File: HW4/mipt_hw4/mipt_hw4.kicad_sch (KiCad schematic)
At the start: 8 parts, among them K1 Panasonic_ALFG1PF12, Q1 BC327, SW1 SW_MEC_5E

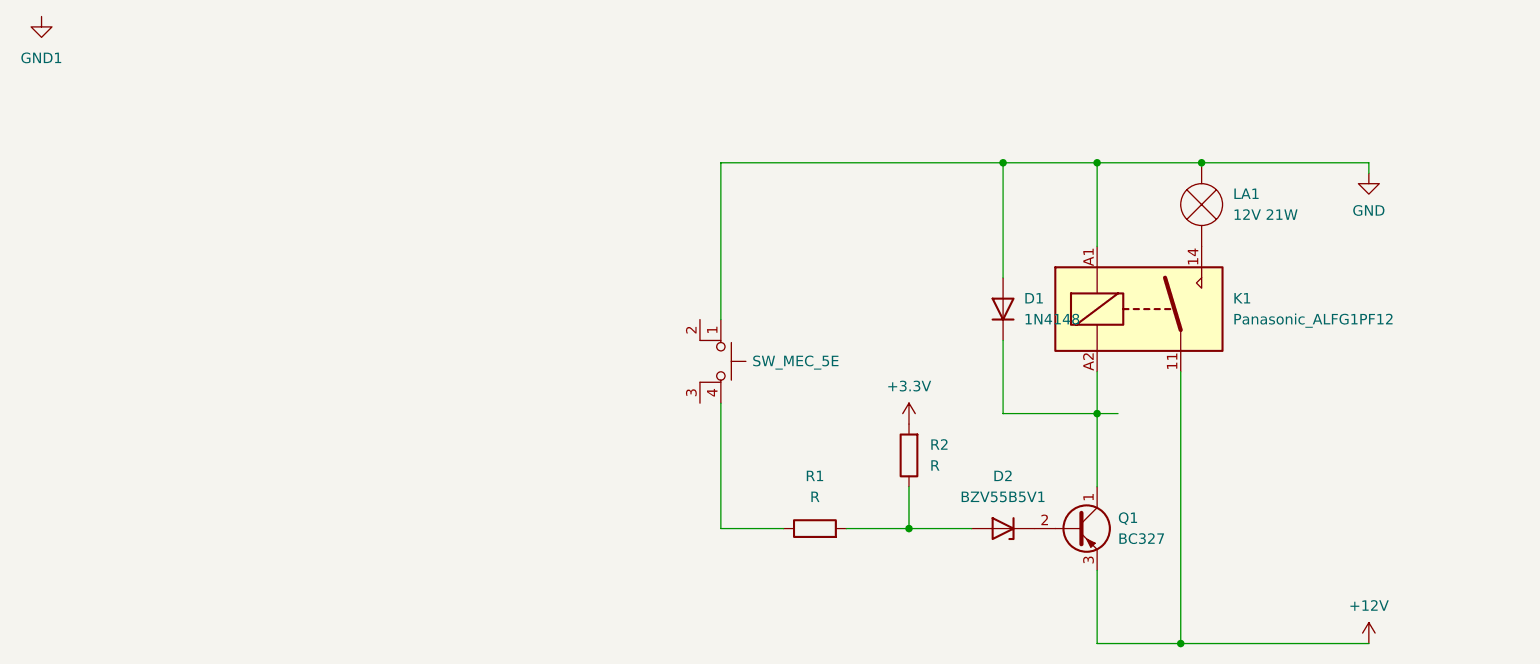
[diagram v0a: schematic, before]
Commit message: HW4 completed
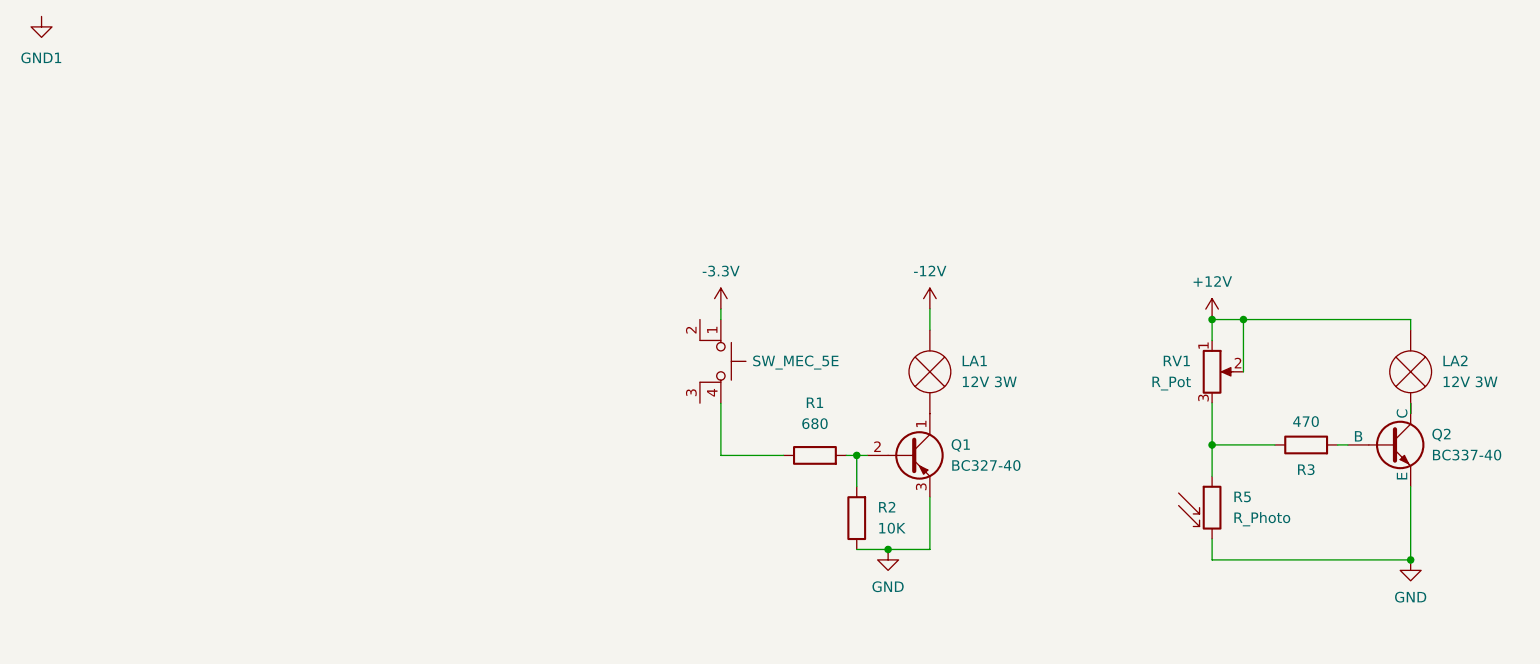
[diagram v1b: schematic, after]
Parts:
- removed D1: 1N4148, Diode_THT:D_DO-35_SOD27_P7.62mm_Horizontal, symbol Diode:1N4148
- removed D2: BZV55B5V1, Diode_SMD:D_MiniMELF, symbol Diode:BZV55B5V1
- removed K1: Panasonic_ALFG1PF12, Relay_THT:Relay_SPST_Panasonic_ALFG_FormA_CircularHoles, symbol Relay:Panasonic_ALFG1PF12
- added LA2: 12V 3W, symbol Device:Lamp
- added Q2: BC337-40, symbol Simulation_SPICE:NPN
- added R3: 470, symbol Device:R
- added R5: R_Photo, symbol Device:R_Photo
- added RV1: R_Pot, symbol Device:R_Potentiometer
- LA1: value 12V 21W -> 12V 3W
- Q1: value BC327 -> BC327-40
- R1: value R -> 680
- R2: value R -> 10K
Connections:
- net +3.3V is gone; now on an unnamed net: R2.2
- net +12V: now also LA2.2 (+), RV1.1, RV1.2; no longer Q1.3 (E)
- net GND: now also Q1.3 (E), R2.1, Q2.3 (E), R5.2; no longer LA1.2 (+), SW1.1
- net at Q1.2 (B): now also R1.2
- net at Q1.1 (C): now also LA1.1 (-)
- new net: R3.1, R5.1, RV1.3
- new net: Q2.2 (B), R3.2
- new net: LA2.1 (-), Q2.1 (C)
- new net -12V: LA1.2 (+)
- new net -3.3V: SW1.1
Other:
- moved on the sheet: LA1, Q1, R1, R2
